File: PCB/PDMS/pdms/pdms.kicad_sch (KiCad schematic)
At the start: 55 parts, among them IC19 STM32L496ZGT6, IC20 AT25SF128A-SHB-T, J1 DBG, J2 6473427-1, J3 N01_036_6501_001, J4 DBG, J5 SAFETY, Y1 16Mhz, Y2 32KHz

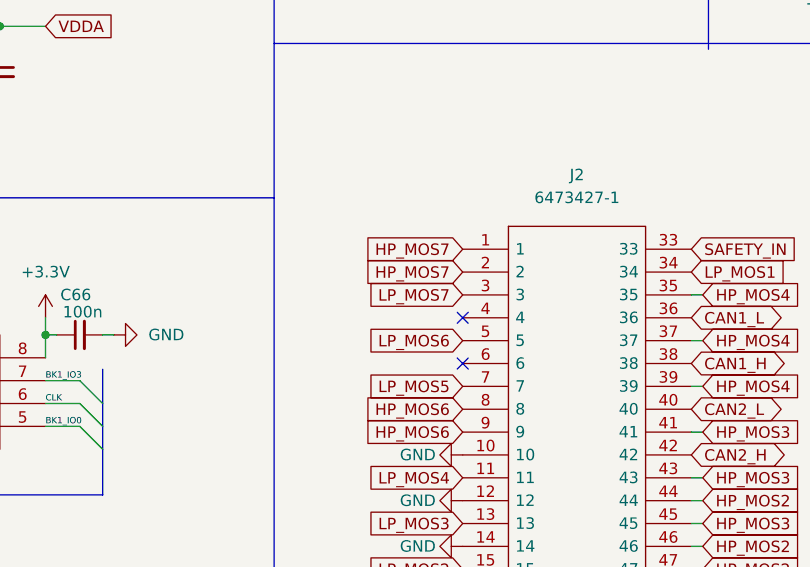
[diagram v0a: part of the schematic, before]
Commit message: Sitched via side
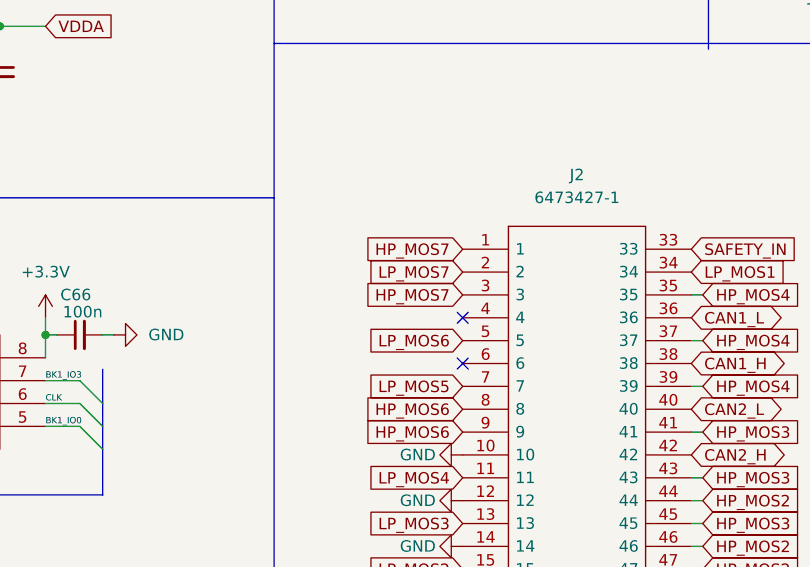
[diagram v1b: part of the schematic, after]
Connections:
- net HP_MOS7: now also J2.3; no longer J2.2
- net LP_MOS7: now also J2.2; no longer J2.3
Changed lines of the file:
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@@
     )
   )
-  (global_label "HP_MOS7" (shape input) (at 332.105 159.385 180) (fields_autoplaced)
+  (global_label "HP_MOS7" (shape input) (at 332.105 161.925 180) (fields_autoplaced)
     (effects (font (size 1.27 1.27)) (justify right))
-    (property "Intersheet References" "${INTERSHEET_REFS}" (id 0) (at 320.9229 159.3056 0)
+    (property "Intersheet References" "${INTERSHEET_REFS}" (id 0) (at 320.9229 161.8456 0)
       (effects (font (size 1.27 1.27)) (justify right) hide)
     )
@@
     )
   )
-  (global_label "LP_MOS7" (shape input) (at 332.105 161.925 180) (fields_autoplaced)
+  (global_label "LP_MOS7" (shape input) (at 332.105 159.385 180) (fields_autoplaced)
     (effects (font (size 1.27 1.27)) (justify right))
-    (property "Intersheet References" "${INTERSHEET_REFS}" (id 0) (at 321.2252 161.8456 0)
+    (property "Intersheet References" "${INTERSHEET_REFS}" (id 0) (at 321.2252 159.3056 0)
       (effects (font (size 1.27 1.27)) (justify right) hide)
     )
@@
       (reference "#PWR0378") (unit 1) (value "+5V") (footprint "")
     )
+    (path "/5e0d1f91-4fae-411e-a2b8-95f4b4fcadc5/a440236e-372c-41e7-add7-4b8781296e41"
+      (reference "#PWR0379") (unit 1) (value "GND") (footprint "")
+    )
     (path "/c4ca1078-fd8d-4af6-b44e-00e6aed0cd5e"
       (reference "#PWR0380") (unit 1) (value "GND") (footprint "")
@@
     )
     (path "/5e0d1f91-4fae-411e-a2b8-95f4b4fcadc5/50334e3e-f97b-45b1-a00b-5148d7178b01"
-      (reference "#PWR?") (unit 1) (value "+5V") (footprint "")
-    )
-    (path "/5e0d1f91-4fae-411e-a2b8-95f4b4fcadc5/a440236e-372c-41e7-add7-4b8781296e41"
-      (reference "#PWR?") (unit 1) (value "GND") (footprint "")
+      (reference "#PWR0383") (unit 1) (value "+5V") (footprint "")
     )
     (path "/12a3a5c1-ac79-4586-9274-31138d63f5db/afc75a69-04d1-4636-8ea3-b3fe3061a65f"
@@
       (reference "R168") (unit 1) (value "1.2k") (footprint "Resistor_SMD:R_0402_1005Metric")
     )
-    (path "/5e0d1f91-4fae-411e-a2b8-95f4b4fcadc5/064f68cd-33aa-440f-a561-ea7f56e641ba"
-      (reference "R?") (unit 1) (value "1k") (footprint "Resistor_SMD:R_0402_1005Metric")
-    )
     (path "/5e0d1f91-4fae-411e-a2b8-95f4b4fcadc5/e56fe53b-8d81-47aa-bdfc-2ba550736a36"
-      (reference "R?") (unit 1) (value "1k") (footprint "Resistor_SMD:R_0402_1005Metric")
+      (reference "R169") (unit 1) (value "1k") (footprint "Resistor_SMD:R_0402_1005Metric")
+    )
+    (path "/5e0d1f91-4fae-411e-a2b8-95f4b4fcadc5/064f68cd-33aa-440f-a561-ea7f56e641ba"
+      (reference "R170") (unit 1) (value "1k") (footprint "Resistor_SMD:R_0402_1005Metric")
     )
     (path "/b84c6964-5564-4d57-8b96-ee4462f76a3a"
